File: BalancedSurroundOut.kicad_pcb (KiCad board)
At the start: 2 copper layers, 48 x 73 mm, 63 parts, among them IC1 TPS61252DSGT, IC2 DRV135UA_2K5, IC3 DRV135UA_2K5, J1 Conn_02x10_Odd_Even, J2 Conn_01x02, J3 XLR3_Ground, J4 XLR3_Ground, J5 Conn_01x03, J6 Conn_01x02, J8 Conn_01x03, U1 LM27762, U2 PCM5102, U3 TLV75533PDBV

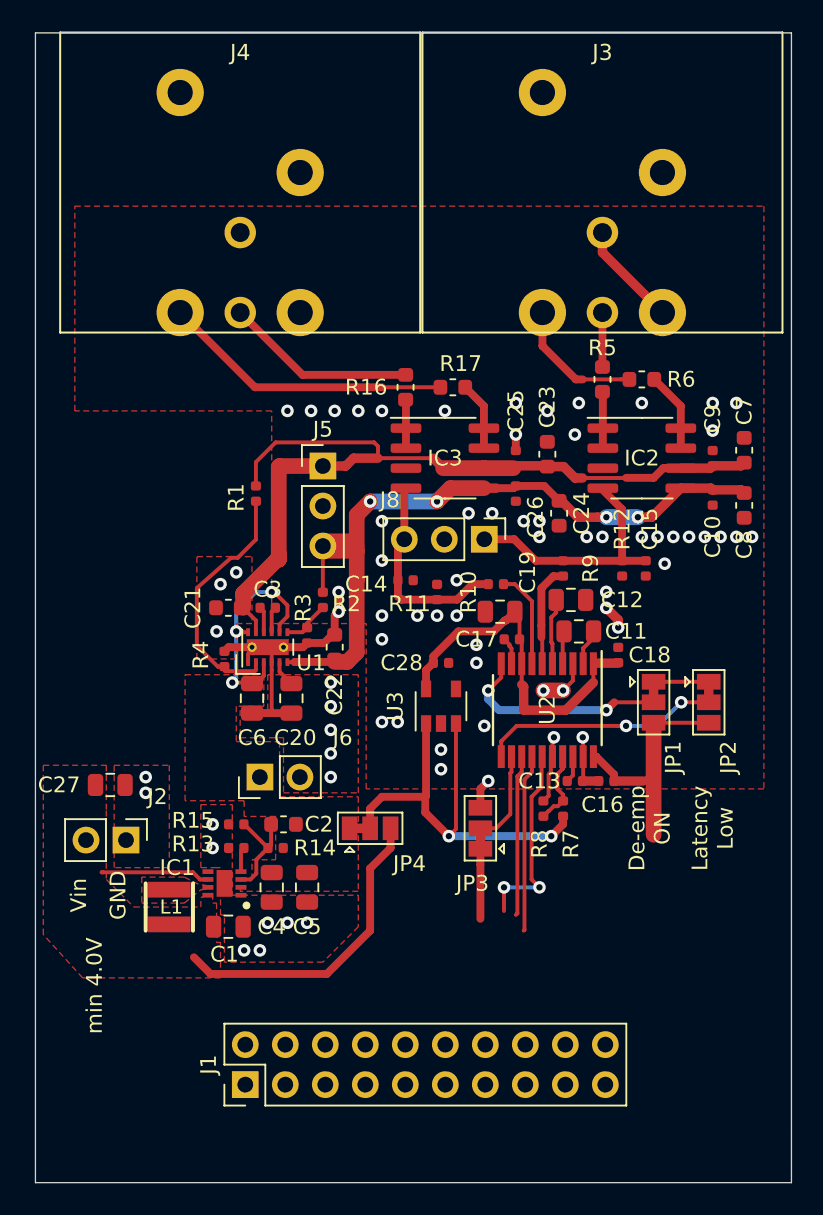
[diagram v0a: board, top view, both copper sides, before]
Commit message: refactor
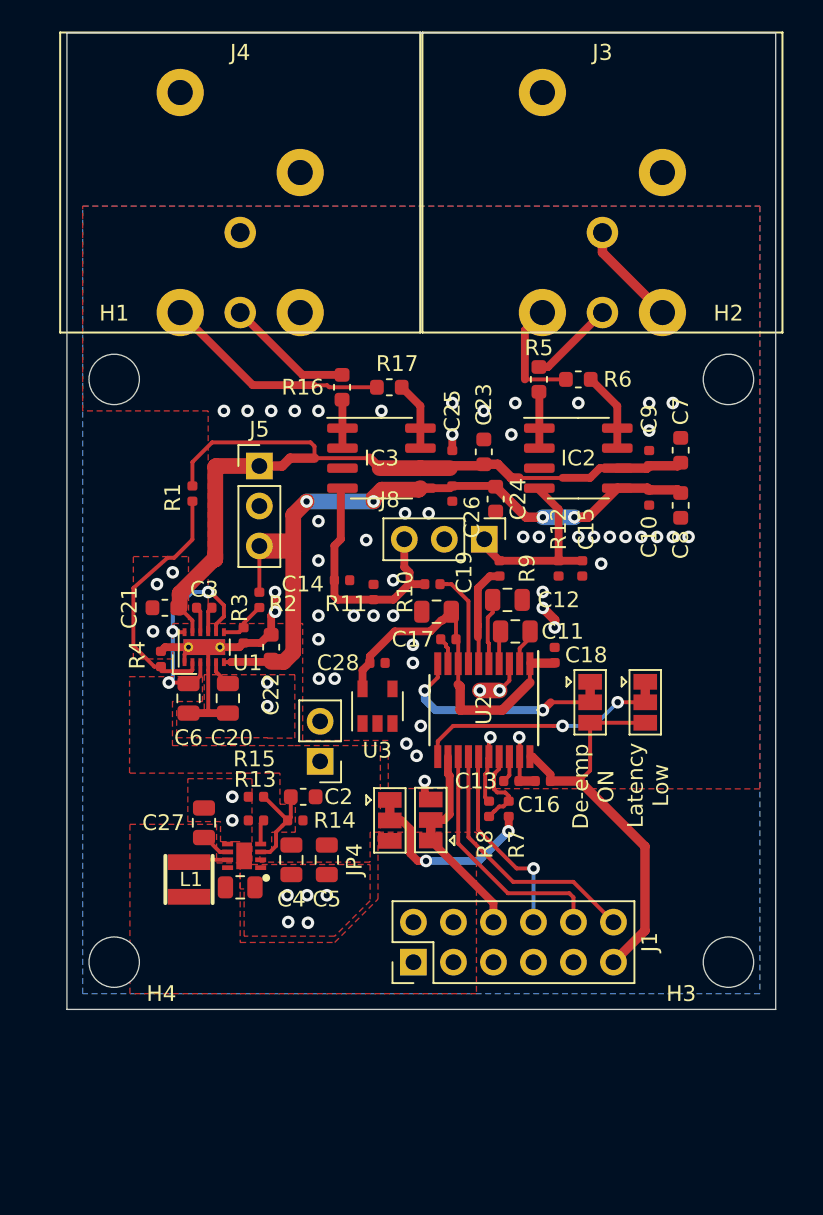
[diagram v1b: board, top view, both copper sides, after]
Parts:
- removed J2: Conn_01x02, Connector_PinHeader_2.54mm:PinHeader_1x02_P2.54mm_Vertical
- added H1: MountingHole, MountingHole:MountingHole_3.2mm_M3, F.Cu at (148.0, 85.0)
- added H2: MountingHole, MountingHole:MountingHole_3.2mm_M3, F.Cu at (187.0, 85.0)
- added H3: MountingHole, MountingHole:MountingHole_3.2mm_M3, F.Cu at (187.0, 122.0)
- added H4: MountingHole, MountingHole:MountingHole_3.2mm_M3, F.Cu at (148.0, 122.0)
- J1: value Conn_02x10_Odd_Even -> Conn_02x06_Odd_Even; footprint Connector_PinHeader_2.54mm:PinHeader_2x10_P2.54mm_Vertical -> Connector_PinHeader_2.54mm:PinHeader_2x06_P2.54mm_Vertical
- moved J1 13.2 mm to (167.0, 122.0)
- moved C27 6.42 mm to (153.7, 113.2), turned to 90 degrees
- moved C24 4.13 mm to (172.2, 92.6)
- moved C23 4.04 mm to (171.5, 89.6)
- moved R10 4.03 mm to (168.2, 98.0)
- moved C10 4.03 mm to (182.0, 92.5)
- moved C11 4.03 mm to (173.5, 101.0)
- moved C12 4.03 mm to (173.0, 99.0)
- moved C13 4.03 mm to (173.2, 110.5)
- moved C14 4.03 mm to (162.5, 97.8)
- moved C15 4.03 mm to (177.7, 97.0)
- moved C16 4.03 mm to (175.2, 110.5)
- moved C17 4.03 mm to (169.2, 101.5)
- moved C18 4.03 mm to (176.0, 102.5)
- moved C19 4.03 mm to (168.5, 99.8)
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- renumbered JP3 to locked
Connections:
- J1 pad 1: /F3 -> VIN
- J1 pad 10: /MCLK -> /BCLK
- J1 pad 11: GND -> +3V3
- J1 pad 12: /LRCLK -> /DIN
- J1 pad 3: /F2 -> VIN
- J1 pad 4: +3V3 -> /DOUT
- J1 pad 5: /F1 -> unconnected-(J1-Pad5)
- J1 pad 6: GND -> /MCLK
- J1 pad 7: /F0 -> GND
- J1 pad 8: /DSDOE -> /LRCLK
- J1 pad 9: /D64 -> GND
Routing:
- net VIN: track 26.8 -> 1.14 mm
- net Net-(JP4-Pad2): track 28.3 -> 11.2 mm
- net +3V3: track 18.6 -> 25.5 mm
- net /BCLK: track 10.2 -> 15.8 mm
- net /DIN: track 11.3 -> 16.6 mm
- net GND: track 48.0 -> 43.6 mm, vias 73 -> 66
- net Net-(J4-Pad2): track 18.5 -> 14.4 mm
- net Net-(J4-Pad3): track 12.1 -> 8.11 mm
- net /DAC/LEFT: track 15.8 -> 12.0 mm
- net /DAC/RIGHT: track 13.3 -> 16.3 mm
- net /PowerSupply/SWITCH: track 0.00 -> 2.51 mm
- net /MCLK: track 4.45 -> 6.83 mm
- net Net-(J3-Pad3): track 3.46 -> 5.46 mm
- net Net-(J3-Pad2): track 8.52 -> 7.31 mm
- net /DAC/MCLK: track 5.95 -> 5.06 mm
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- added copper zone on B.Cu, net GND
- removed copper zone on F.Cu, net /PowerSupply/SWITCH
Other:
- board size 48 x 73 mm -> 45 x 62 mm
- board text removed: "GND"
- board text removed: "Vin"
- board text removed: "min 4.0V"
